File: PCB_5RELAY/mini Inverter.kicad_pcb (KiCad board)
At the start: 2 copper layers, 103.6 x 77.8 mm, 38 parts, among them IC1 ULN2003, J1 Conn_01x05_Pin, J2 Conn_01x03_Pin, U1 HLK-PM12, U2 L7805, U3 AMS1117, U5 ESP32-WROOM-32E

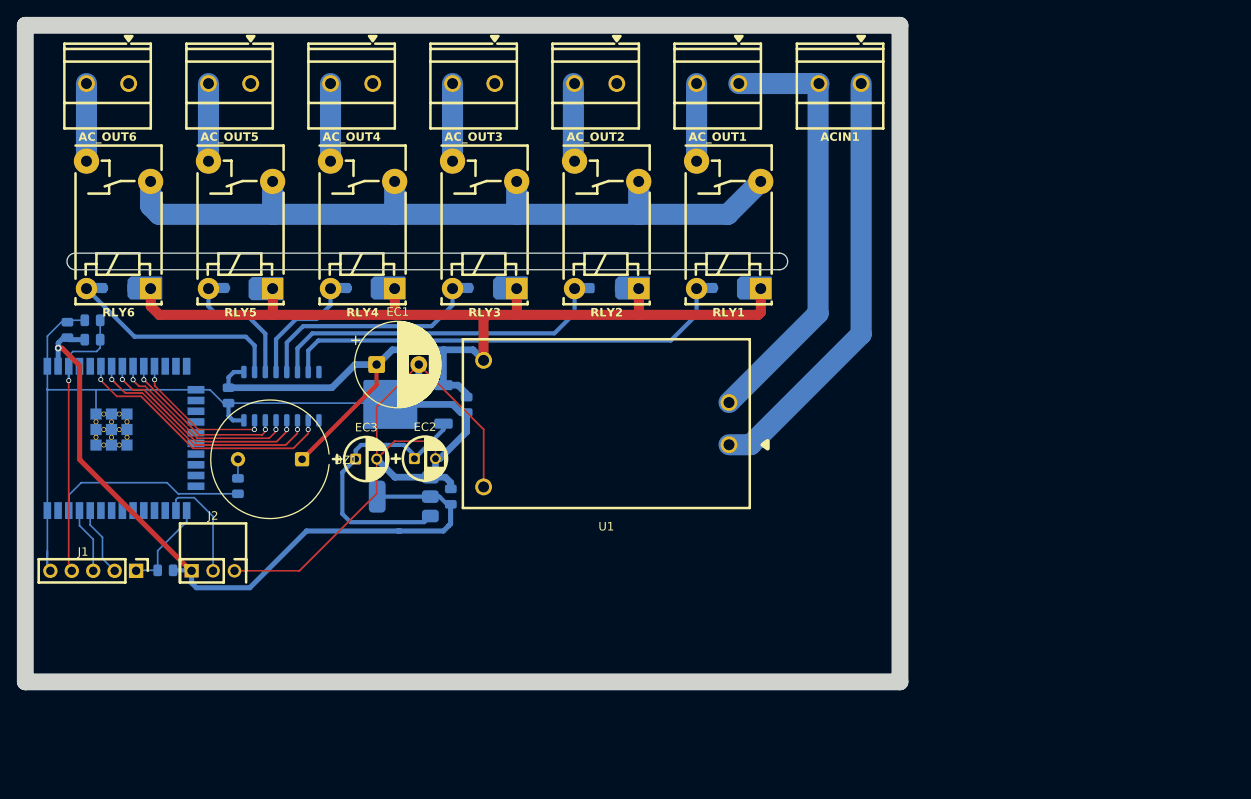
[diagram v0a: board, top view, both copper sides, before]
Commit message: 151026
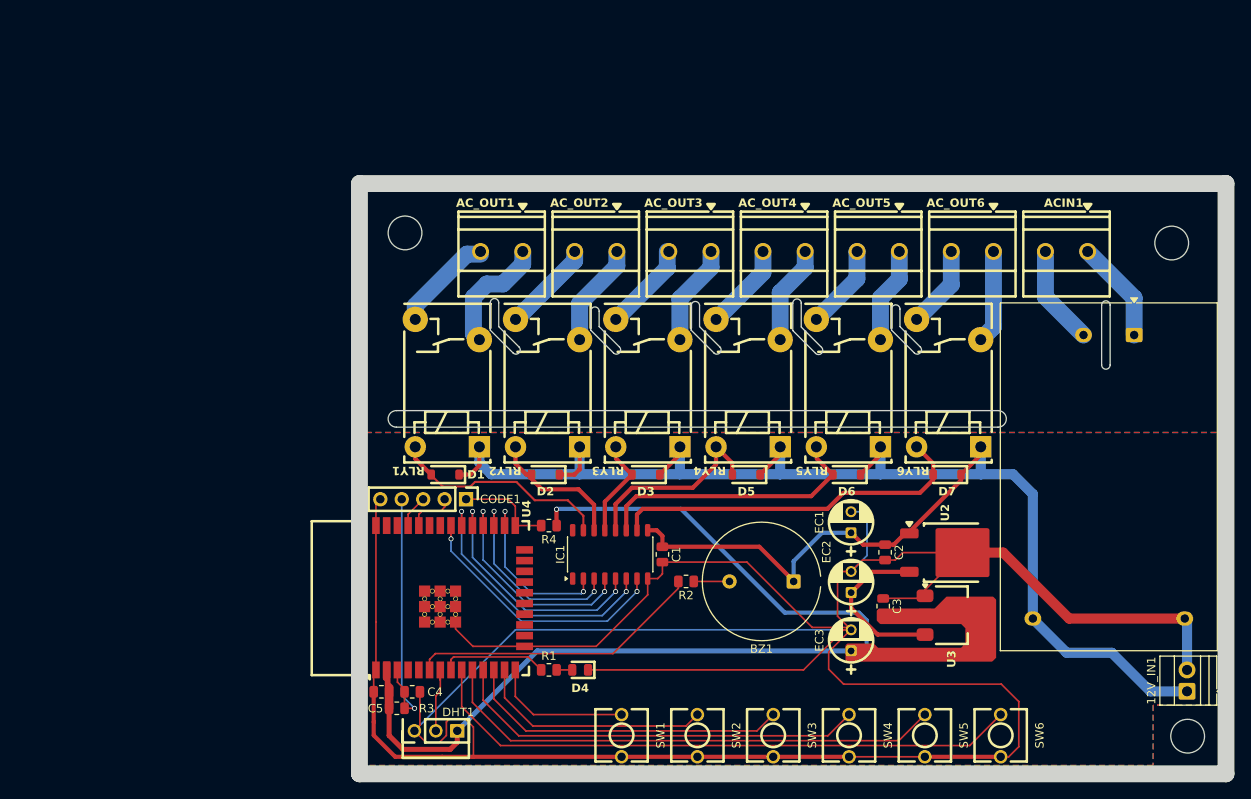
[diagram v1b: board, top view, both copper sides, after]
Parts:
- added 12V_IN1: Conn_01x02_Pin, TerminalBlock:TerminalBlock_Xinya_XY308-2.54-2P_1x02_P2.54mm_Horizontal, F.Cu at (193.9, 130.0)
- added ?: , clipboard:7b5fcdc5-8954-4c17-bed2-f8229795bd91, F.Cu at (101.2, 75.7)
- added ?: , clipboard:7b5fcdc5-8954-4c17-bed2-f8229795bd91, F.Cu at (192.1, 76.9)
- added ?: , clipboard:7b5fcdc5-8954-4c17-bed2-f8229795bd91, F.Cu at (194.0, 135.3)
- added D4: LED, 1_Mycustomfootprint:LED_0805_2012Metric, F.Cu at (122.0, 127.5)
- added R1: 10K, Resistor_SMD:R_0805_2012Metric, F.Cu at (118.3, 127.5)
- added SW1: Nút Nhấn 6x6mm Cao 5.5mm 2 Chân, 1_Mycustomfootprint:Nút Nhấn 6x6mm Cao 5.5mm, F.Cu at (126.9, 135.2)
- added SW2: Nút Nhấn 6x6mm Cao 5.5mm 2 Chân, 1_Mycustomfootprint:Nút Nhấn 6x6mm Cao 5.5mm, F.Cu at (135.9, 135.2)
- added SW3: Nút Nhấn 6x6mm Cao 5.5mm 2 Chân, 1_Mycustomfootprint:Nút Nhấn 6x6mm Cao 5.5mm, F.Cu at (144.9, 135.2)
- added SW4: Nút Nhấn 6x6mm Cao 5.5mm 2 Chân, 1_Mycustomfootprint:Nút Nhấn 6x6mm Cao 5.5mm, F.Cu at (153.9, 135.2)
- added SW5: Nút Nhấn 6x6mm Cao 5.5mm 2 Chân, 1_Mycustomfootprint:Nút Nhấn 6x6mm Cao 5.5mm, F.Cu at (162.8, 135.2)
- added SW6: Nút Nhấn 6x6mm Cao 5.5mm 2 Chân, 1_Mycustomfootprint:Nút Nhấn 6x6mm Cao 5.5mm, F.Cu at (171.8, 135.2)
- C1: renamed from C4; moved to F.Cu
- C2: renamed from C1; value 0805 -> 104; moved to F.Cu
- C3: renamed from C2; value 0805 -> 104; moved to F.Cu
- C4: renamed from C5; moved to F.Cu
- C5: renamed from C3; moved to F.Cu
- D1: renamed from D6; footprint Diode_SMD:D_SOD-123 -> 1_Mycustomfootprint:D_SOD-123; moved to F.Cu
- D2: renamed from D5; footprint Diode_SMD:D_SOD-123 -> 1_Mycustomfootprint:D_SOD-123; moved to F.Cu
- D3: renamed from D4; footprint Diode_SMD:D_SOD-123 -> 1_Mycustomfootprint:D_SOD-123; moved to F.Cu
- D5: renamed from D3; footprint Diode_SMD:D_SOD-123 -> 1_Mycustomfootprint:D_SOD-123; moved to F.Cu
- D6: renamed from D2; footprint Diode_SMD:D_SOD-123 -> 1_Mycustomfootprint:D_SOD-123; moved to F.Cu
- D7: renamed from D1; footprint Diode_SMD:D_SOD-123 -> 1_Mycustomfootprint:D_SOD-123; moved to F.Cu
- EC1: value C_Polarized -> 220µF/25V; footprint Capacitor_THT:CP_Radial_D10.0mm_P5.00mm -> 1_Mycustomfootprint:CP_Radial_D5.0mm_P2.50mm
- EC2: value C_Polarized -> 47µF
- EC3: value C_Polarized -> 10µF
- IC1: moved to F.Cu
- R2: renamed from R4; moved to F.Cu
- R3: renamed from R5; moved to F.Cu
- R4: renamed from R6; moved to F.Cu
- U1: value HLK-PM12 -> HLK-10M-12 (10W); footprint 1_Mycustomfootprint:Converter_ACDC_Hi-Link_HLK-PMxx -> Converter_ACDC:Converter_ACDC_Hi-Link_HLK-5Mxx
- U2: footprint Package_TO_SOT_SMD:TO-252-2 -> 1_Mycustomfootprint:TO-252-2; moved to F.Cu
- U3: footprint Package_TO_SOT_SMD:SOT-223-3_TabPin2 -> 1_Mycustomfootprint:SOT-223-3_TabPin2; moved to F.Cu
- U4: renamed from U5; moved to F.Cu
- moved U2 66.8 mm to (165.2, 113.6), turned to -90 degrees
- moved U3 66.4 mm to (166.0, 121.0), turned to -90 degrees
- moved U1 63.4 mm to (187.7, 87.8), turned to -90 degrees
- moved EC3 61.4 mm to (154.1, 124.0), turned to 90 degrees
- moved BZ1 60.0 mm to (147.3, 117.0)
- moved EC1 59.2 mm to (154.1, 110.0), turned to 90 degrees
- moved C4 58.1 mm to (102.1, 130.1), turned to 0 degrees
- moved C5 56.8 mm to (98.5, 130.1), turned to 180 degrees
- moved R3 56.6 mm to (100.3, 132.0)
- moved C1 54.8 mm to (131.8, 113.8)
- moved R2 54.3 mm to (134.6, 117.0), turned to 180 degrees
- moved C3 52.9 mm to (157.9, 119.9)
- moved EC2 52.6 mm to (154.1, 117.1), turned to 90 degrees
- moved C2 52.6 mm to (158.1, 113.6)
- moved AC_OUT1 50.8 mm to (112.7, 77.9)
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- renumbered AC_OUT6 to AC_OUT1, AC_OUT5 to AC_OUT2, AC_OUT4 to AC_OUT3, AC_OUT3 to AC_OUT4, AC_OUT2 to AC_OUT5, AC_OUT1 to AC_OUT6, J1 to CODE1, J2 to DHT1, RLY6 to RLY1, RLY5 to RLY2, RLY4 to RLY3, RLY3 to RLY4, RLY2 to RLY5, RLY1 to RLY6
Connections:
- net /AC_RL1 renamed /ACOUT61
- net /AC_RL2 renamed /ACOUT51
- net /AC_RL3 renamed /ACOUT41
- net /AC_RL4 renamed /ACOUT31
- net /AC_RL5 renamed /ACOUT21
- net /AC_RL6 renamed /ACOUT11
- AC_OUT1 pad 1: /ACN -> /ACOUT12
- AC_OUT2 pad 1: /ACN -> /ACOUT22
- AC_OUT3 pad 1: /ACN -> /ACOUT32
- AC_OUT4 pad 1: /ACN -> /ACOUT42
- AC_OUT5 pad 1: /ACN -> /ACOUT52
- AC_OUT6 pad 1: /ACN -> /ACOUT62
- EC3 pad 1: +5V -> +3V3
- IC1 pad 10: /O6 -> /O1
- IC1 pad 11: /O5 -> /O2
- IC1 pad 12: /O4 -> /O3
- IC1 pad 13: /O3 -> /O4
- IC1 pad 14: /O2 -> /O5
- IC1 pad 15: /O1 -> /O6
- IC1 pad 2: /IN6 -> /IN1
- IC1 pad 3: /IN5 -> /IN2
- IC1 pad 4: /IN4 -> /IN3
- IC1 pad 5: /IN3 -> /IN4
- IC1 pad 6: /IN2 -> /IN5
- IC1 pad 7: /IN1 -> /IN6
- RLY1 pad 11: /ACN -> /ACOUT12
- RLY2 pad 11: /ACN -> /ACOUT22
- RLY3 pad 11: /ACN -> /ACOUT32
- RLY4 pad 11: /ACN -> /ACOUT42
- RLY5 pad 11: /ACN -> /ACOUT52
- RLY6 pad 11: /ACN -> /ACOUT62
- U4 pad 10: /IN2 -> /BT2
- U4 pad 11: /IN1 -> /BT3
- U4 pad 12: unconnected-(U5-IO27-Pad12) -> /BT4
- U4 pad 13: unconnected-(U5-IO14-Pad13) -> /BT5
- U4 pad 14: unconnected-(U5-IO12-Pad14) -> /BT6
- U4 pad 26: /DHT11 -> /IN1
- U4 pad 27: unconnected-(U5-IO16-Pad27) -> /IN2
- U4 pad 28: unconnected-(U5-IO17-Pad28) -> /IN3
- U4 pad 29: unconnected-(U5-IO5-Pad29) -> /IN4
- U4 pad 30: unconnected-(U5-IO18-Pad30) -> /IN5
- U4 pad 31: unconnected-(U5-IO19-Pad31) -> /IN6
- U4 pad 36: /BUZZ -> unconnected-(U4-IO22-Pad36)
- U4 pad 6: /IN6 -> /BUZZ
- U4 pad 7: /IN5 -> /DHT11
- U4 pad 8: /IN4 -> /LED
- U4 pad 9: /IN3 -> /BT1
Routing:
- net GND: track 184.8 -> 387.7 mm
- net /ACN: track 144.6 -> 11.8 mm
- net /BT1: track 0.00 -> 71.7 mm
- net /BT2: track 0.00 -> 60.6 mm
- net +3V3: track 91.5 -> 145.2 mm
- net /BT3: track 0.00 -> 49.7 mm
- net +12V: track 155.8 -> 198.1 mm
- net /BT4: track 0.00 -> 38.9 mm
- net /ACL: track 50.8 -> 12.2 mm
- net /BT5: track 0.00 -> 28.1 mm
- net /BT6: track 0.00 -> 16.6 mm
- net /ACOUT12: track 0.00 -> 14.3 mm
- net +5V: track 33.0 -> 19.8 mm
- net /LED: track 0.00 -> 12.7 mm
- net /ACOUT22: track 0.00 -> 12.3 mm
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- added copper zone on B.Cu, net GND
- added copper zone on F.Cu, net GND
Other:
- board size 103.6 x 77.8 mm -> 102.7 x 70 mm
